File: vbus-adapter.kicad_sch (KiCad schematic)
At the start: 34 parts, among them J1 VBUS, J2 CAN, J3 Screw_Terminal_01x03, J4 Screw_Terminal_01x03, J6 Backup GPIO, T800 AO3400A, U1 ISO7721FDR, U3 MCP2562-E-SN, U4 WeMos_S2_mini

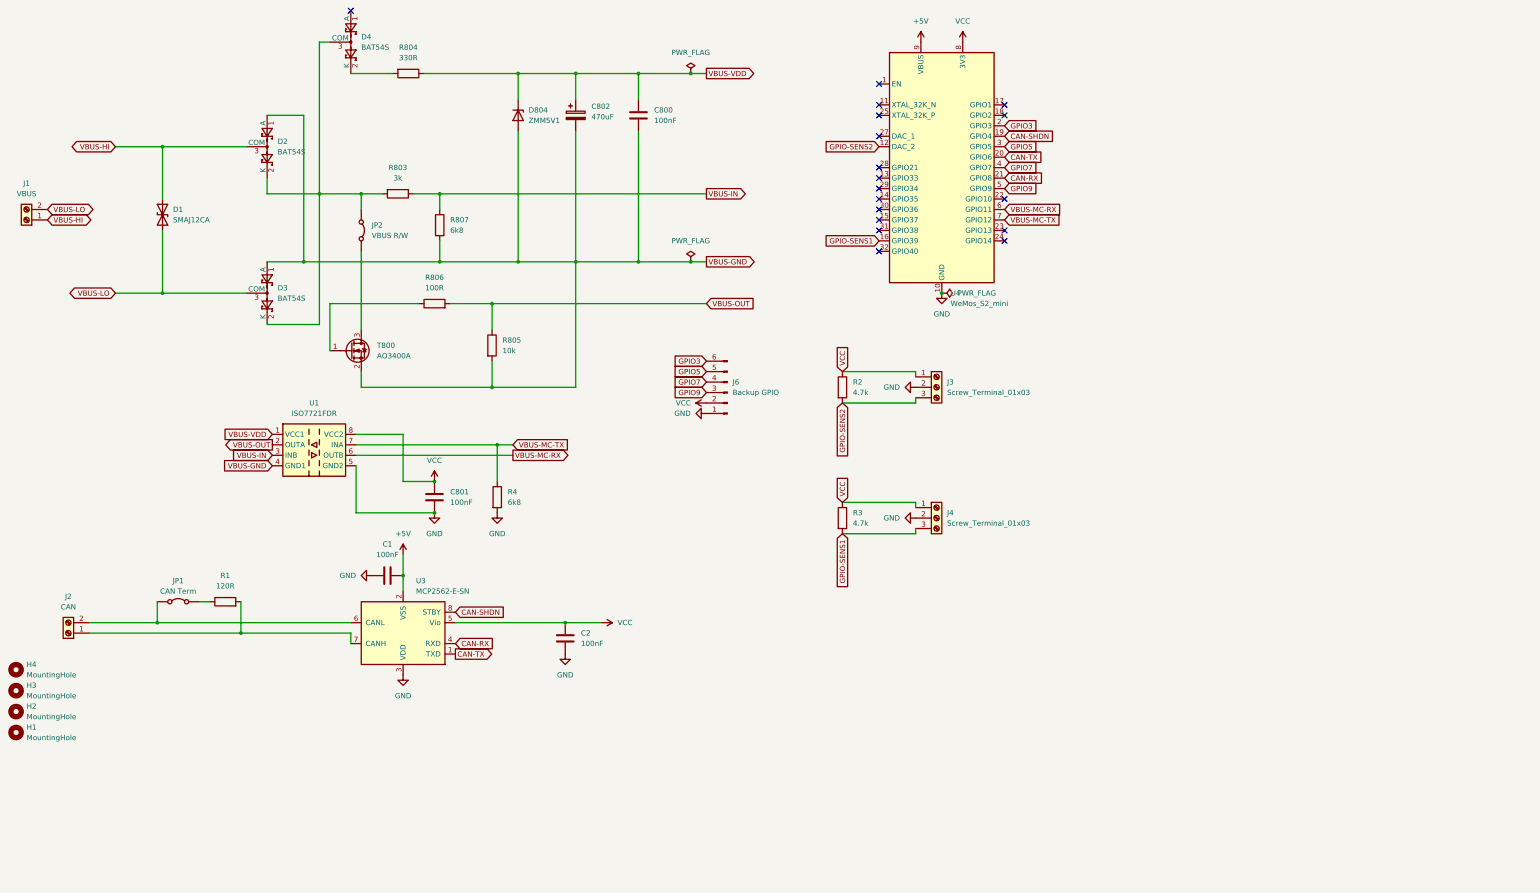
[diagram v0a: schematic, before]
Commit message: Version 2
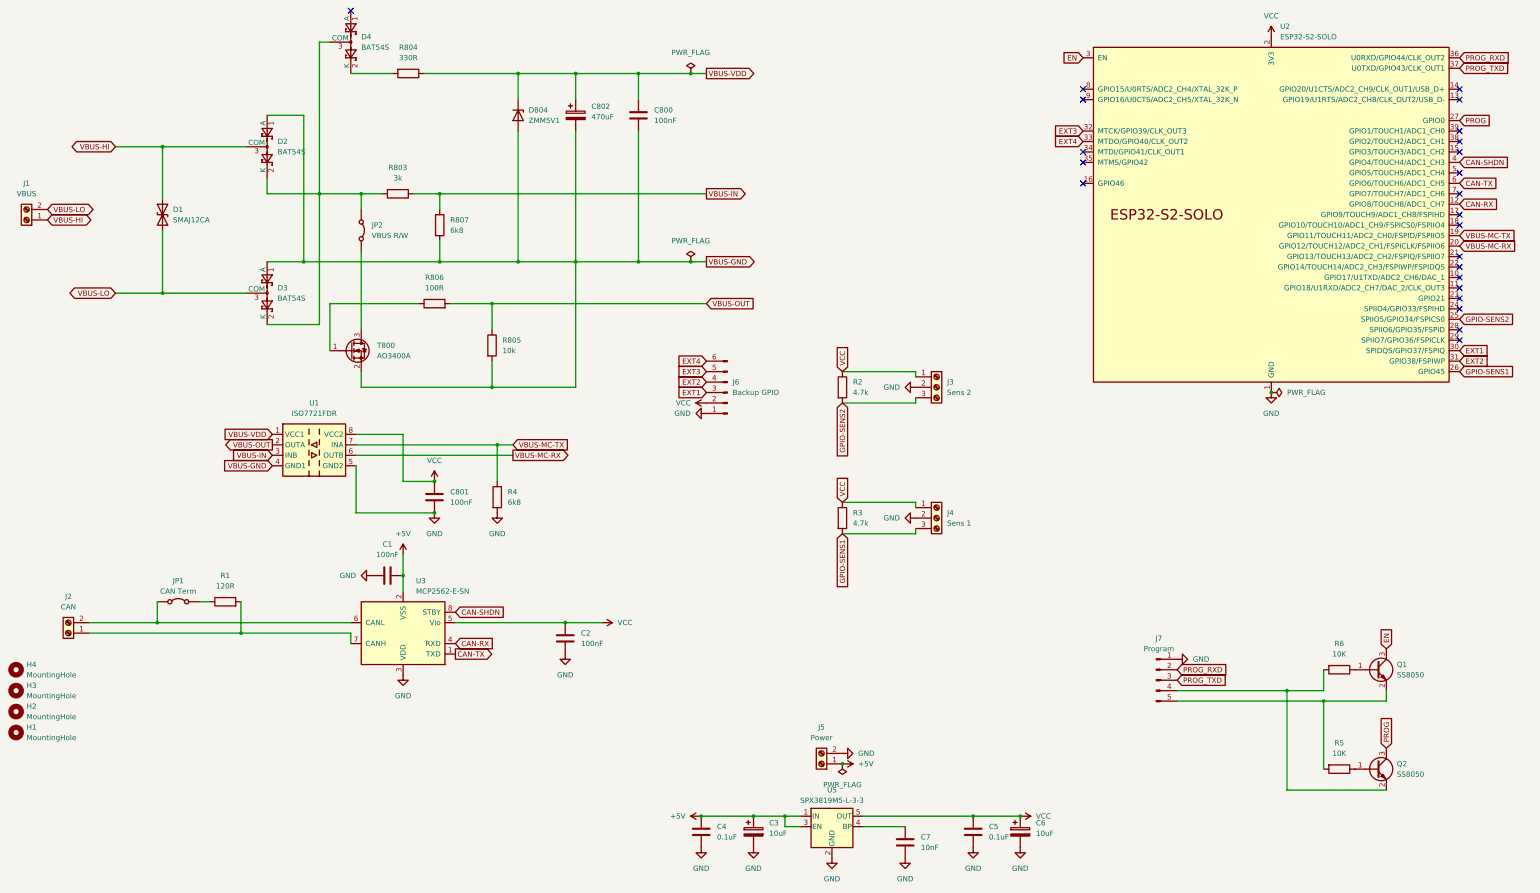
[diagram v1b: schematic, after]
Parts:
- removed U4: WeMos_S2_mini, flo:WEMOS_S2_mini, symbol WEMOS_S2_mini:WeMos_S2_mini
- added C3, C6: 10uF, Capacitor_SMD:C_0805_2012Metric_Pad1.18x1.45mm_HandSolder, symbol Device:C_Polarized
- added C4, C5: 0.1uF, Capacitor_SMD:C_0805_2012Metric_Pad1.18x1.45mm_HandSolder, symbol Device:C
- added C7: 10nF, Capacitor_SMD:C_0805_2012Metric_Pad1.18x1.45mm_HandSolder, symbol Device:C
- added J5: Power, TerminalBlock_Phoenix:TerminalBlock_Phoenix_MPT-0,5-2-2.54_1x02_P2.54mm_Horizontal, symbol Connector:Screw_Terminal_01x02
- added J7: Program, Connector_PinHeader_2.54mm:PinHeader_1x05_P2.54mm_Vertical, symbol Connector:Conn_01x05_Pin
- added Q1, Q2: SS8050, Package_TO_SOT_SMD:SOT-23, symbol Transistor_BJT:SS8050
- added R5, R6: 10K, Resistor_SMD:R_0805_2012Metric_Pad1.20x1.40mm_HandSolder, symbol Device:R
- added U2: ESP32-S2-SOLO, PCM_Espressif:ESP32-S2-SOLO, symbol PCM_Espressif:ESP32-S2-SOLO
- added U5: SPX3819M5-L-3-3, Package_TO_SOT_SMD:SOT-23-5, symbol Regulator_Linear:SPX3819M5-L-3-3
- J1, J2: footprint TerminalBlock_Phoenix:TerminalBlock_Phoenix_MKDS-1,5-2-5.08_1x02_P5.08mm_Horizontal -> TerminalBlock_Phoenix:TerminalBlock_Phoenix_MPT-0,5-2-2.54_1x02_P2.54mm_Horizontal
- J3: value Screw_Terminal_01x03 -> Sens 2; footprint TerminalBlock_Phoenix:TerminalBlock_Phoenix_MKDS-1,5-3-5.08_1x03_P5.08mm_Horizontal -> TerminalBlock_Phoenix:TerminalBlock_Phoenix_MPT-0,5-3-2.54_1x03_P2.54mm_Horizontal
- J4: value Screw_Terminal_01x03 -> Sens 1; footprint TerminalBlock_Phoenix:TerminalBlock_Phoenix_MKDS-1,5-3-5.08_1x03_P5.08mm_Horizontal -> TerminalBlock_Phoenix:TerminalBlock_Phoenix_MPT-0,5-3-2.54_1x03_P2.54mm_Horizontal
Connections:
- net +5V: now also C3.1, C4.1, J5.1 (Pin_1), U5.1 (IN), U5.3 (EN)
- net CAN-RX: now also U2.12 (GPIO8/TOUCH8/ADC1_CH7)
- net CAN-SHDN: now also U2.4 (GPIO4/TOUCH4/ADC1_CH3)
- net CAN-TX: now also U2.6 (GPIO6/TOUCH6/ADC1_CH5)
- net GND: now also C3.2, C4.2, C5.2, C6.2, C7.2, J5.2 (Pin_2), J7.1 (Pin_1), U2.1 (GND), U2.40 (GND), U2.41 (GND), U5.2 (GND)
- net GPIO-SENS1: now also U2.26 (GPIO45)
- net GPIO-SENS2: now also U2.25 (SPIIO5/GPIO34/FSPICS0)
- net VBUS-MC-RX: now also U2.20 (GPIO12/TOUCH12/ADC2_CH1/FSPICLK/FSPIIO6)
- net VBUS-MC-TX: now also U2.19 (GPIO11/TOUCH11/ADC2_CH0/FSPID/FSPIIO5)
- net VCC: now also C5.1, C6.1, U2.2 (3V3), U5.5 (OUT)
- net GPIO3 renamed EXT4
- net EXT4: now also U2.33 (MTDO/GPIO40/CLK_OUT2)
- net GPIO5 renamed EXT3
- net EXT3: now also U2.32 (MTCK/GPIO39/CLK_OUT3)
- net GPIO7 renamed EXT2
- net EXT2: now also U2.31 (GPIO38/FSPIWP)
- net GPIO9 renamed EXT1
- net EXT1: now also U2.30 (SPIDQS/GPIO37/FSPIQ)
- new net: J7.4 (Pin_4), Q2.2 (E), R6.2
- new net: J7.5 (Pin_5), Q1.2 (E), R5.2
- new net: C7.1, U5.4 (BP)
- new net: Q1.1 (B), R6.1
- new net: Q2.1 (B), R5.1
- new net EN: Q1.3 (C), U2.3 (EN)
- new net PROG: Q2.3 (C), U2.27 (GPIO0)
- new net PROG_RXD: J7.2 (Pin_2), U2.36 (U0RXD/GPIO44/CLK_OUT2)
- new net PROG_TXD: J7.3 (Pin_3), U2.37 (U0TXD/GPIO43/CLK_OUT1)
- no-connect marks 18 -> 23
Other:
- title: (none) -> vbus-adapter
